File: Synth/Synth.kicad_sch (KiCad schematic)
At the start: 2 parts, among them U11 LM321, U12 LM321

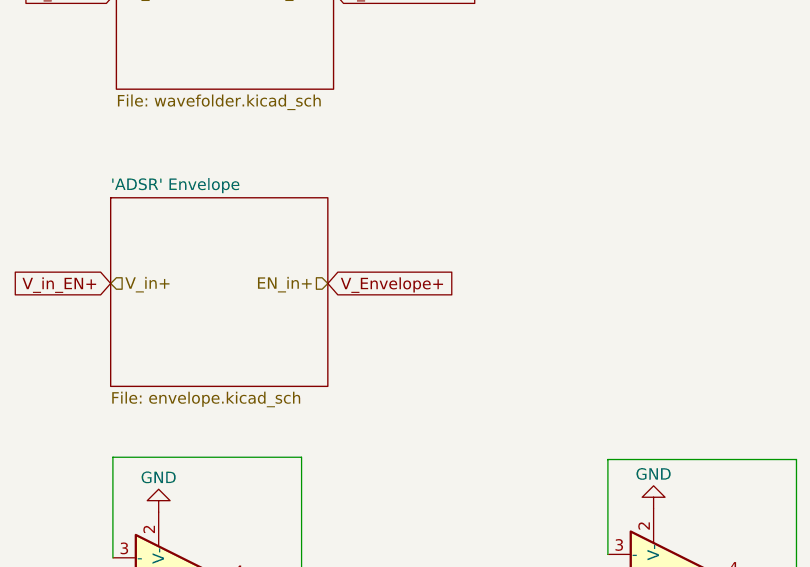
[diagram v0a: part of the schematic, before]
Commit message: add the layout
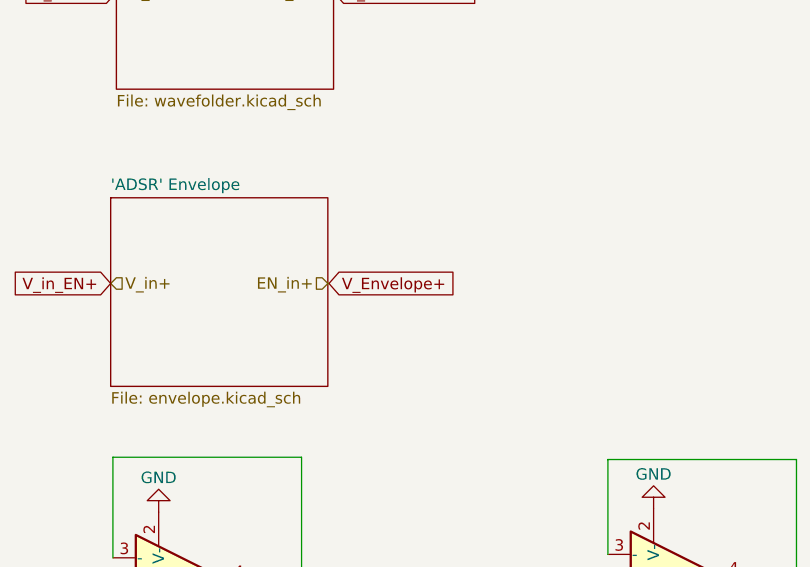
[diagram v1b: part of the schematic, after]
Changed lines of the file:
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@@
+    (stroke (width 0) (type default))
+  )
+  (wire (pts (xy 120.777 72.39) (xy 120.65 72.39))
     (stroke (width 0) (type default))
   )
@@
     )
   )
-  (global_label "V_Envelope+" (shape input) (at 120.65 72.39 0) (fields_autoplaced)
+  (global_label "V_Envelope+" (shape input) (at 120.777 72.39 0) (fields_autoplaced)
     (effects (font (size 1.27 1.27)) (justify left))
-    (property "Intersheetrefs" "${INTERSHEET_REFS}" (at 135.6698 72.39 0)
+    (property "Intersheetrefs" "${INTERSHEET_REFS}" (at 135.7968 72.39 0)
       (effects (font (size 1.27 1.27)) (justify left) hide)
     )
